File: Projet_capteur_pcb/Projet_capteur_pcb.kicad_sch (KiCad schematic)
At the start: 18 parts, among them J1 Power, J2 Digital/PWM, J3 Analog, J4 Digital/PWM

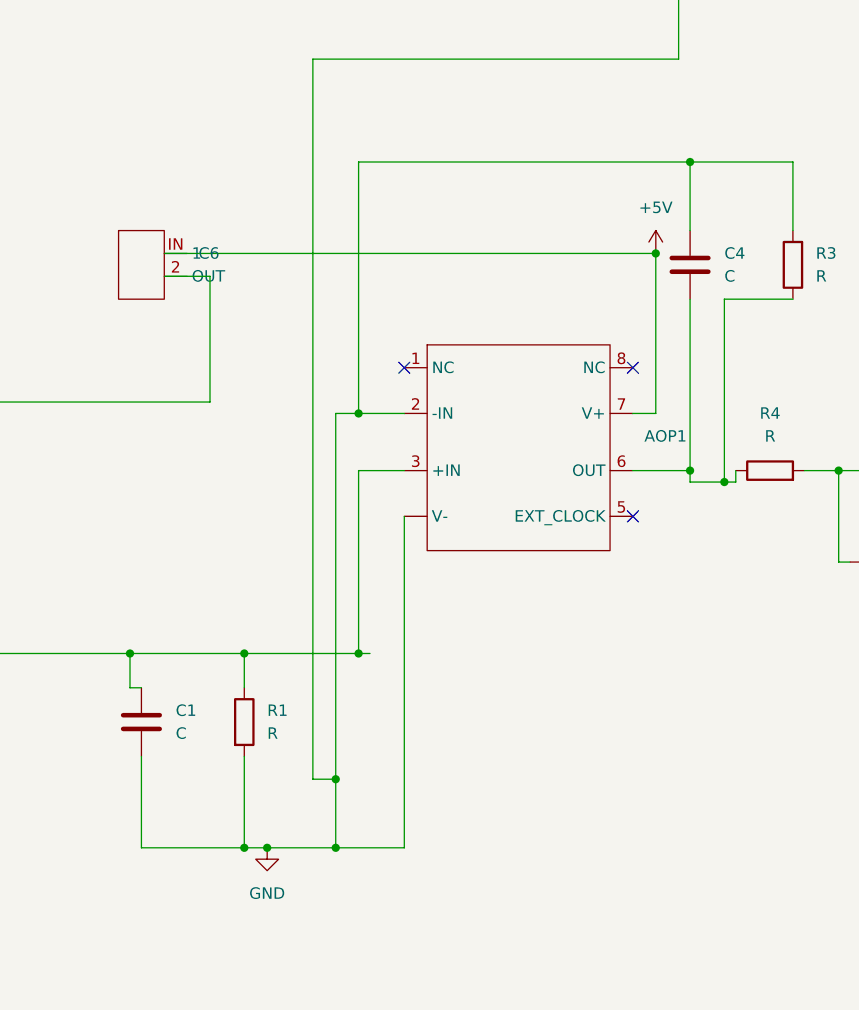
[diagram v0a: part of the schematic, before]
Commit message: routage
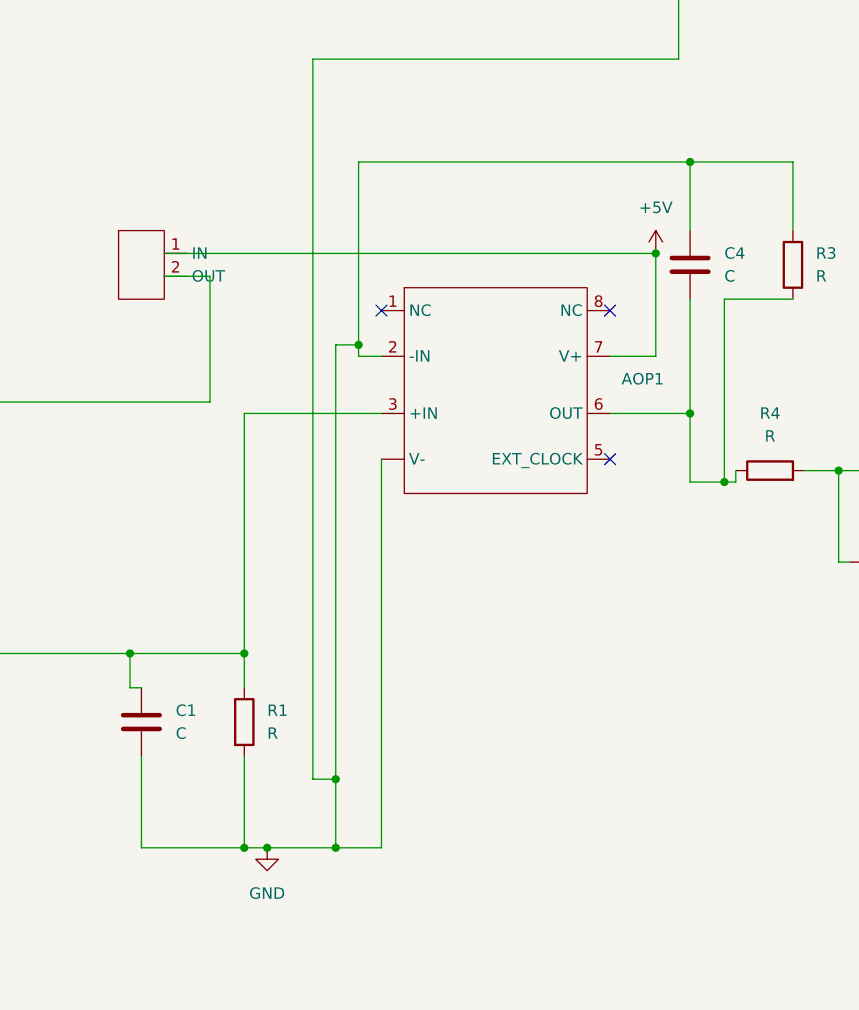
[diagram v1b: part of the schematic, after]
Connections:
- net +5V: now also C6.1 (IN); no longer C6.IN (1)
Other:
- moved on the sheet: AOP1
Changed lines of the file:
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@@
 	)
 	(junction
-		(at 213.36 135.89)
-		(diameter 0)
-		(color 0 0 0 0)
-	)
-	(junction
-		(at 213.36 109.22)
+		(at 250.19 109.22)
 		(diameter 0)
 		(color 0 0 0 0)
@@
 	)
 	(junction
-		(at 200.66 135.89)
-		(diameter 0)
-		(color 0 0 0 0)
-	)
-	(junction
 		(at 266.7 115.57)
 		(diameter 0)
@@
 	)
 	(junction
-		(at 250.19 115.57)
+		(at 200.66 135.89)
+		(diameter 0)
+		(color 0 0 0 0)
+	)
+	(junction
+		(at 213.36 101.6)
 		(diameter 0)
 		(color 0 0 0 0)
@@
 	)
 	(no_connect
-		(at 243.84 120.65)
+		(at 241.3 114.3)
 	)
 	(no_connect
-		(at 218.44 104.14)
+		(at 215.9 97.79)
 	)
 	(no_connect
@@
 	)
 	(no_connect
-		(at 243.84 104.14)
+		(at 241.3 97.79)
 	)
 	(no_connect
@@
 	(wire
 		(pts
-			(xy 243.84 115.57) (xy 250.19 115.57)
+			(xy 241.3 109.22) (xy 250.19 109.22)
 		)
 		(stroke
@@
 	(wire
 		(pts
-			(xy 213.36 135.89) (xy 214.63 135.89)
+			(xy 31.75 44.45) (xy 31.75 46.99)
 		)
 		(stroke
 			(width 0)
-			(type default)
+			(type solid)
 		)
 	)
 	(wire
 		(pts
-			(xy 31.75 44.45) (xy 31.75 46.99)
+			(xy 213.36 81.28) (xy 213.36 101.6)
 		)
 		(stroke
 			(width 0)
-			(type solid)
+			(type default)
 		)
 	)
@@
 	(wire
 		(pts
-			(xy 243.84 109.22) (xy 246.38 109.22)
+			(xy 210.82 101.6) (xy 213.36 101.6)
+		)
+		(stroke
+			(width 0)
+			(type default)
+		)
+	)
+	(wire
+		(pts
+			(xy 241.3 102.87) (xy 246.38 102.87)
 		)
 		(stroke
@@
 	(wire
 		(pts
-			(xy 210.82 157.48) (xy 218.44 157.48)
+			(xy 215.9 157.48) (xy 210.82 157.48)
 		)
 		(stroke
@@
 	(wire
 		(pts
-			(xy 213.36 115.57) (xy 218.44 115.57)
+			(xy 200.66 109.22) (xy 215.9 109.22)
 		)
 		(stroke
@@
 	(wire
 		(pts
-			(xy 250.19 96.52) (xy 250.19 115.57)
+			(xy 250.19 96.52) (xy 250.19 109.22)
 		)
 		(stroke
@@
 	(wire
 		(pts
-			(xy 213.36 109.22) (xy 218.44 109.22)
+			(xy 213.36 102.87) (xy 215.9 102.87)
 		)
 		(stroke
@@
 	(wire
 		(pts
-			(xy 213.36 109.22) (xy 213.36 81.28)
-		)
-		(stroke
-			(width 0)
-			(type default)
-		)
-	)
-	(wire
-		(pts
 			(xy 62.23 67.31) (xy 74.93 67.31)
 		)
@@
 	(wire
 		(pts
-			(xy 246.38 91.44) (xy 246.38 109.22)
+			(xy 246.38 91.44) (xy 246.38 102.87)
 		)
 		(stroke
@@
 	(wire
 		(pts
-			(xy 19.05 34.29) (xy 34.29 34.29)
+			(xy 213.36 101.6) (xy 213.36 102.87)
 		)
 		(stroke
 			(width 0)
-			(type solid)
+			(type default)
 		)
 	)
 	(wire
 		(pts
-			(xy 213.36 115.57) (xy 213.36 135.89)
+			(xy 19.05 34.29) (xy 34.29 34.29)
 		)
 		(stroke
 			(width 0)
-			(type default)
+			(type solid)
 		)
 	)
@@
 	(wire
 		(pts
-			(xy 34.29 46.99) (xy 31.75 46.99)
+			(xy 200.66 135.89) (xy 200.66 109.22)
 		)
 		(stroke
 			(width 0)
-			(type solid)
+			(type default)
 		)
 	)
 	(wire
 		(pts
-			(xy 248.92 69.85) (xy 248.92 52.07)
+			(xy 34.29 46.99) (xy 31.75 46.99)
 		)
 		(stroke
 			(width 0)
-			(type default)
+			(type solid)
 		)
 	)
 	(wire
 		(pts
-			(xy 210.82 109.22) (xy 213.36 109.22)
+			(xy 248.92 69.85) (xy 248.92 52.07)
 		)
 		(stroke
@@
 	(wire
 		(pts
-			(xy 200.66 135.89) (xy 213.36 135.89)
+			(xy 250.19 109.22) (xy 250.19 116.84)
 		)
 		(stroke
@@
 	(wire
 		(pts
-			(xy 250.19 115.57) (xy 250.19 116.84)
-		)
-		(stroke
-			(width 0)
-			(type default)
-		)
-	)
-	(wire
-		(pts
 			(xy 21.59 59.69) (xy 34.29 59.69)
 		)
@@
 	(wire
 		(pts
-			(xy 218.44 120.65) (xy 218.44 157.48)
+			(xy 215.9 114.3) (xy 215.9 157.48)
 		)
 		(stroke
@@
 	(wire
 		(pts
-			(xy 210.82 109.22) (xy 210.82 149.86)
+			(xy 210.82 101.6) (xy 210.82 149.86)
 		)
 		(stroke
@@
 	(symbol
 		(lib_id "Graphique_bluetooth:aop")
-		(at 231.14 113.03 0)
+		(at 228.6 106.68 0)
 		(unit 1)
 		(exclude_from_sim no)
@@
 		(fields_autoplaced yes)
 		(property "Reference" "AOP1"
-			(at 245.11 111.7599 0)
+			(at 242.57 105.4099 0)
 			(effects
 				(font
@@
 		)
 		(property "Value" "~"
-			(at 245.11 114.2999 0)
+			(at 242.57 107.9499 0)
 			(effects
 				(font
@@
 		)
 		(property "Footprint" "Librairie_empreinte:AO"
-			(at 231.14 113.03 0)
+			(at 228.6 106.68 0)
 			(effects
 				(font
@@
 		)
 		(property "Datasheet" ""
-			(at 231.14 113.03 0)
+			(at 228.6 106.68 0)
 			(effects
 				(font
@@
 		)
 		(property "Description" ""
-			(at 231.14 113.03 0)
+			(at 228.6 106.68 0)
 			(effects
 				(font
@@
 				)
 				(justify left)
+				(hide yes)
 			)
 		)
@@
 			)
 		)
-		(pin "IN"
+		(pin "1"
 		)
 		(pin "2"

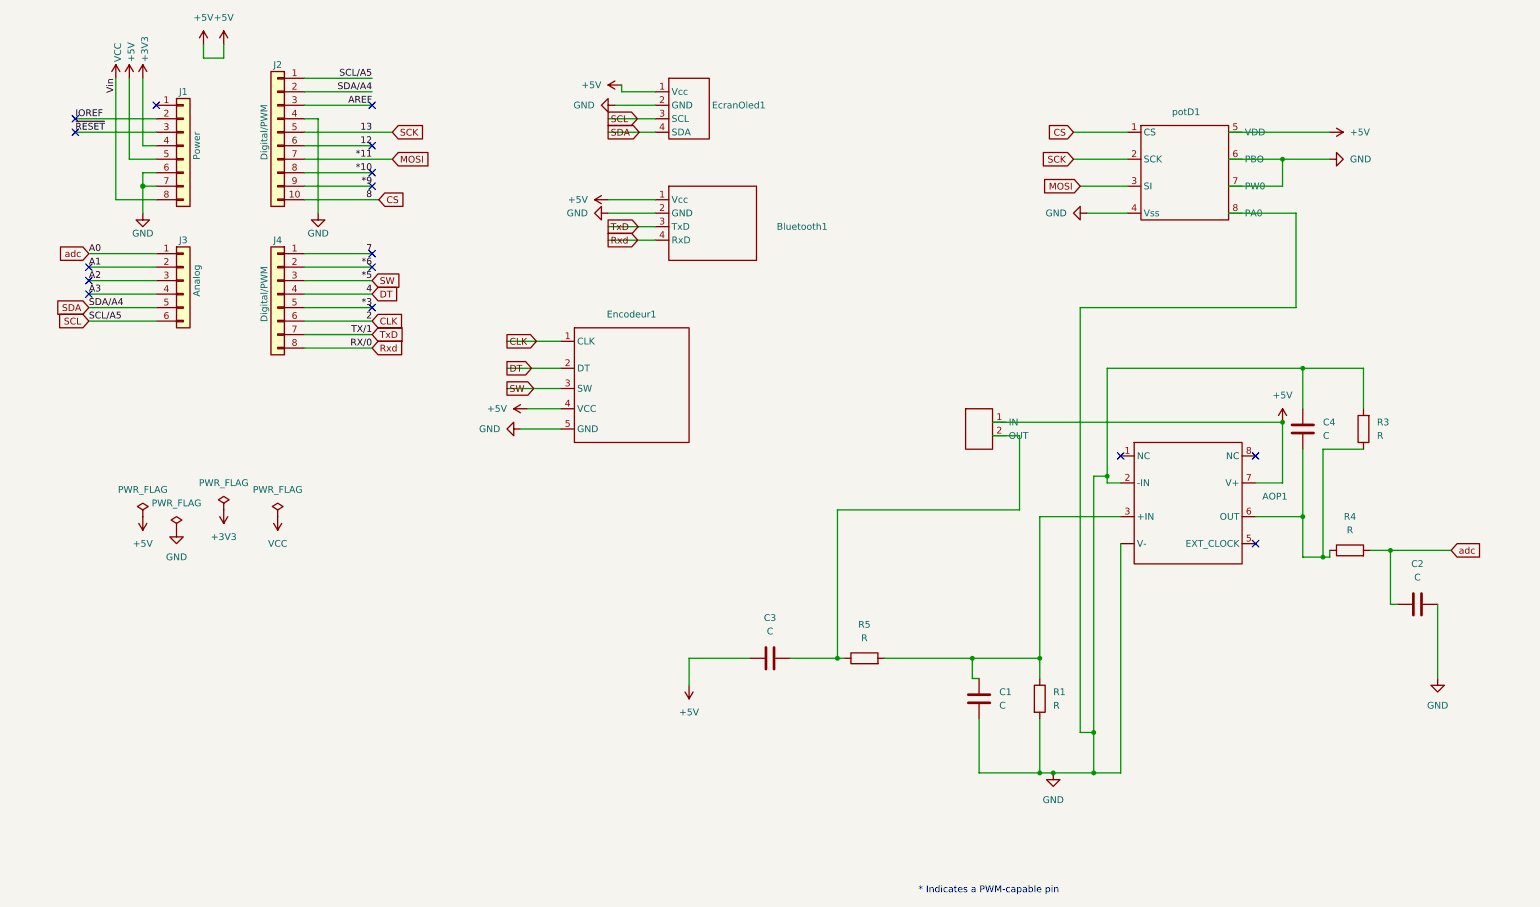
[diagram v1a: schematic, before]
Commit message: routage V1
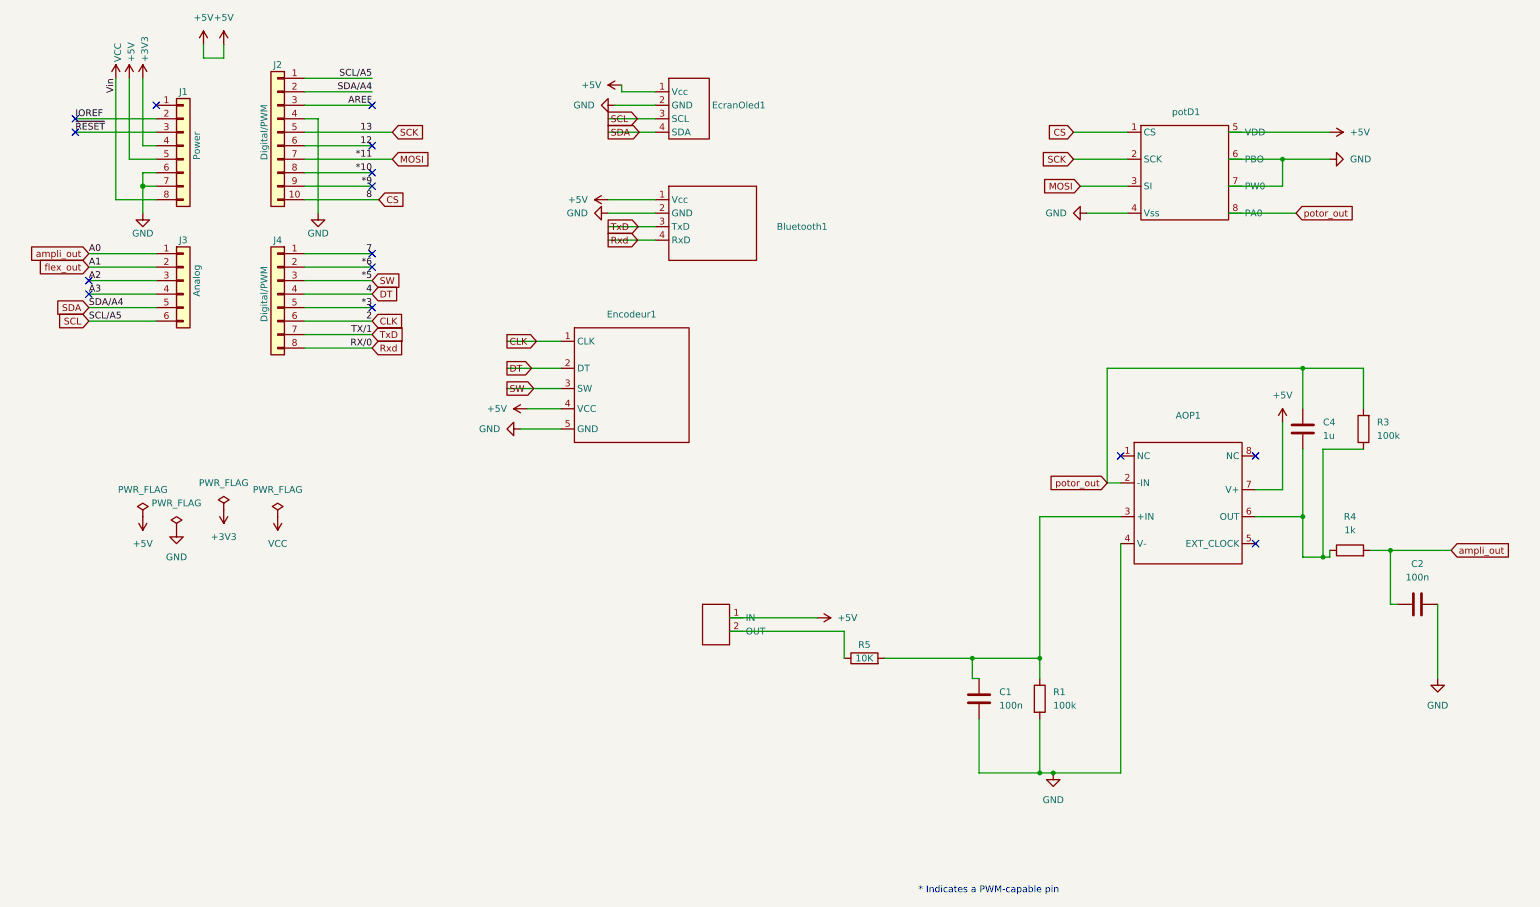
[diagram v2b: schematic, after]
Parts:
- removed C3: C, Capacitor_THT:C_Disc_D7.5mm_W2.5mm_P5.00mm, symbol Device:C
- C1, C2: value C -> 100n
- C4: value C -> 1u
- R1, R3: value R -> 100k
- R4: value R -> 1k
- R5: value R -> 10K
- capteur1: renamed from C6; footprint (none) -> Librairie_empreinte:DIP-2_296_ELL
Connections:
- net GND: now also AOP1.4 (V-); no longer AOP1. (V-), AOP1.2 (-IN), C4.1, R3.2, potD1.8 (PA0)
- net A1 renamed flex_out
- net adc renamed ampli_out
- new net potor_out: AOP1.2 (-IN), C4.1, R3.2, potD1.8 (PA0)
- no-connect marks 16 -> 15
